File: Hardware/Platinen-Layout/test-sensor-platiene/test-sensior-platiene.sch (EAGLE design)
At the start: 38 parts, among them J10 Flash Programming, J5 Flash Programming, U1 AS72651, U10 4MB Flash, U2 4MB Flash, U5 AS72653, U6 AS72652, U9 IR

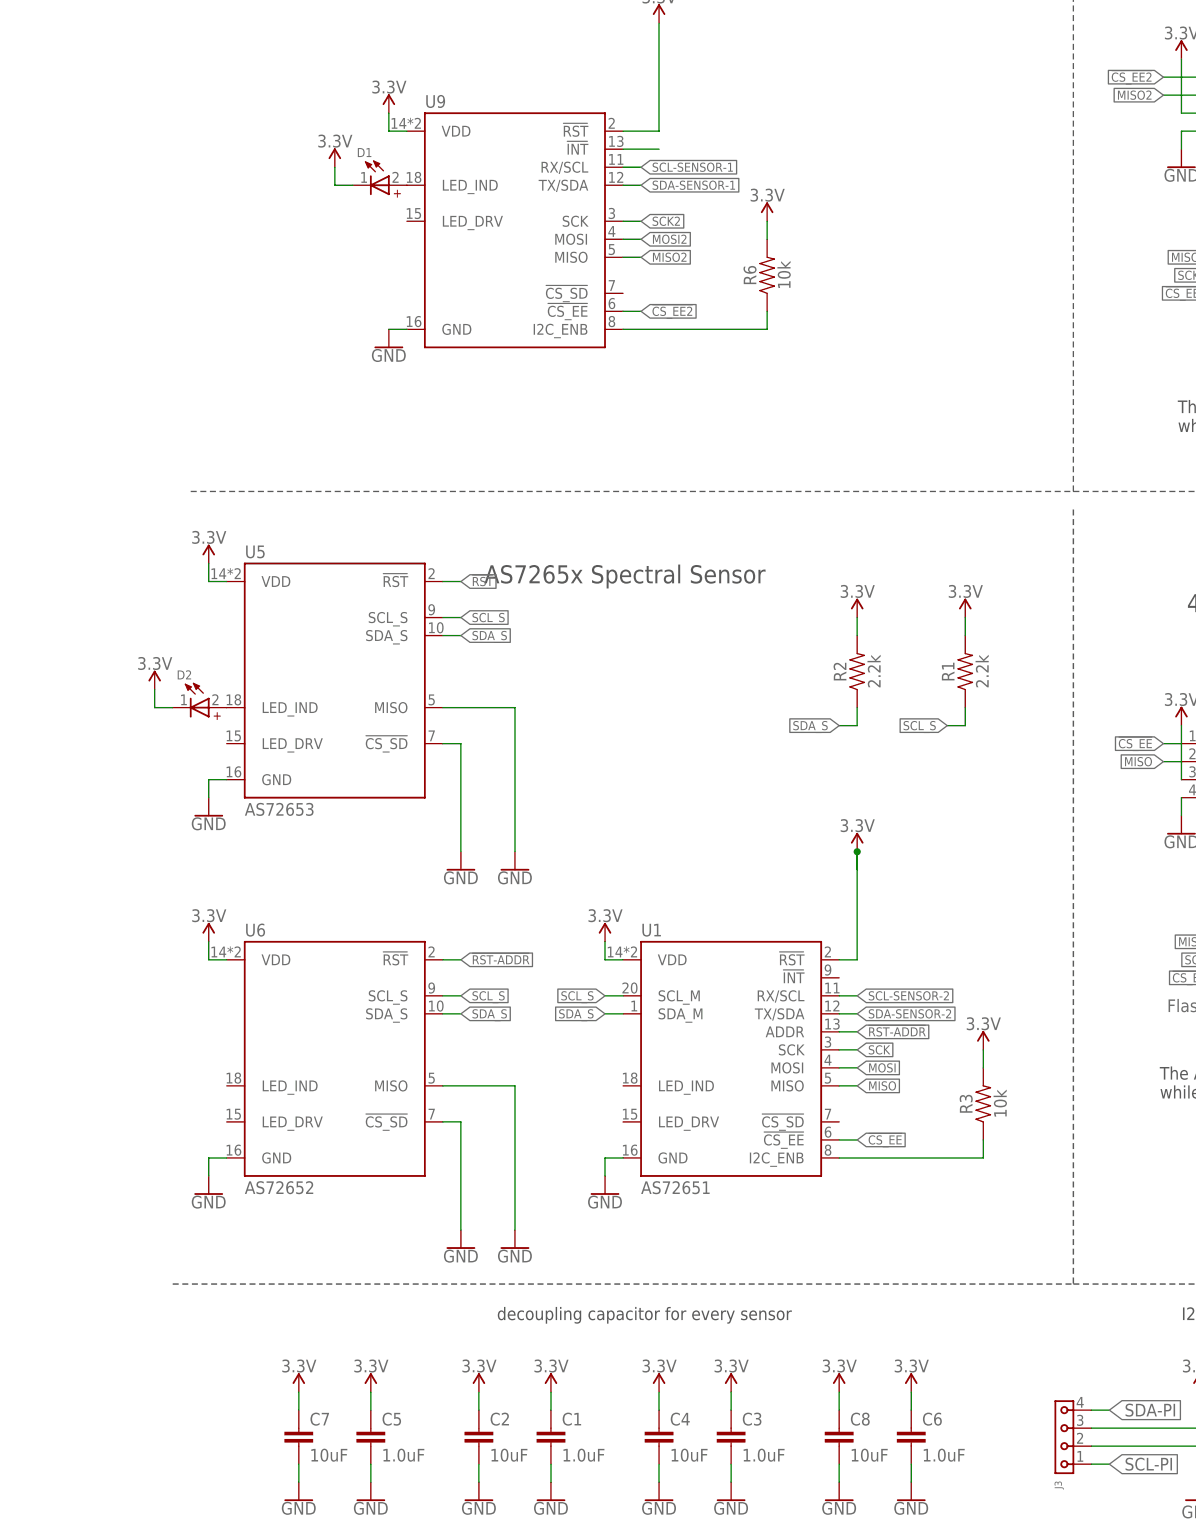
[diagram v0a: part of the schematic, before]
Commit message: board is a mess
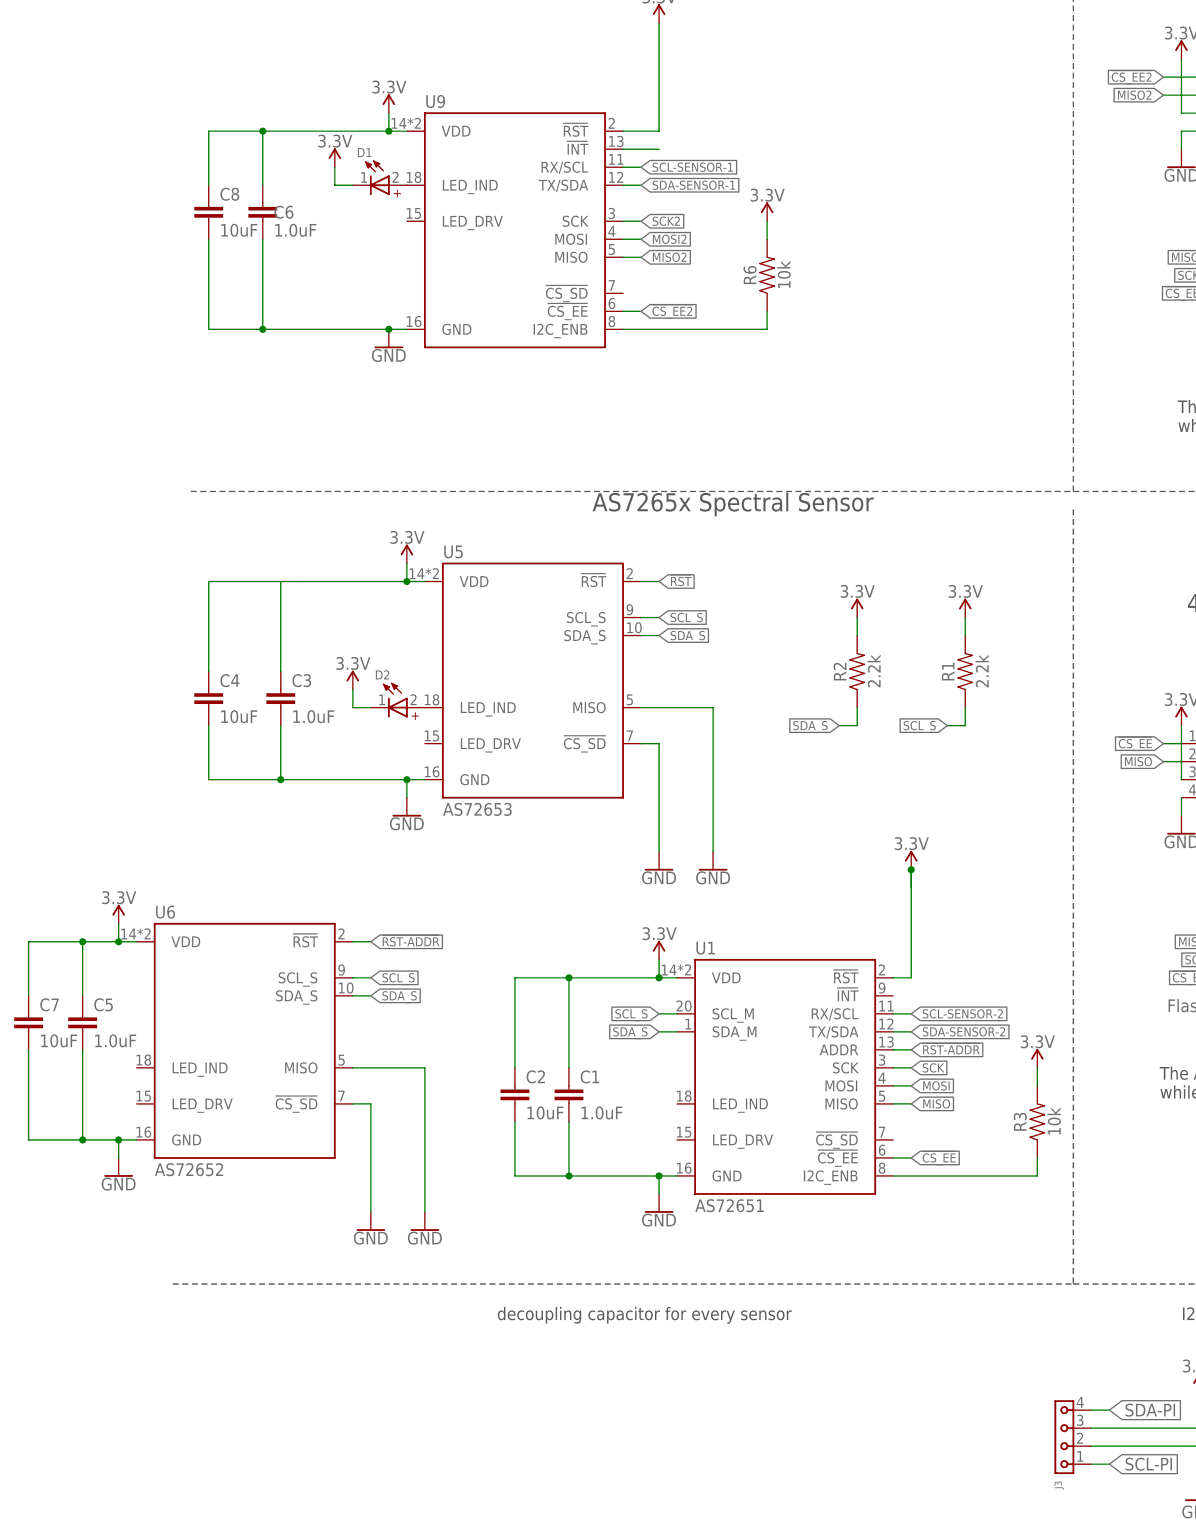
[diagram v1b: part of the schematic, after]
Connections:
- new net N$11: J3.2
- new net N$8: J1.2
- net GND: no longer J1.2, J3.2
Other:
- moved on the sheet: C1, C2, C3, C4, C5, C6, C7, C8, D2, R3, U1, U5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
